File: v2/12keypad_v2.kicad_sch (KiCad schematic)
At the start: 56 parts, among them J1 USB_C_Receptacle_USB2.0, SW1 SW_SPDT, SW10 KEY_MX, SW11 KEY_MX, SW2 KEY_MX, SW3 KEY_MX, SW4 KEY_MX, SW5 KEY_MX, SW6 KEY_MX, SW7 KEY_MX, SW8 KEY_MX, SW9 KEY_MX, U1 RP2040, U2 NCP1117-3.3_SOT223, U3 W25Q128JVS, Y1 12MHz

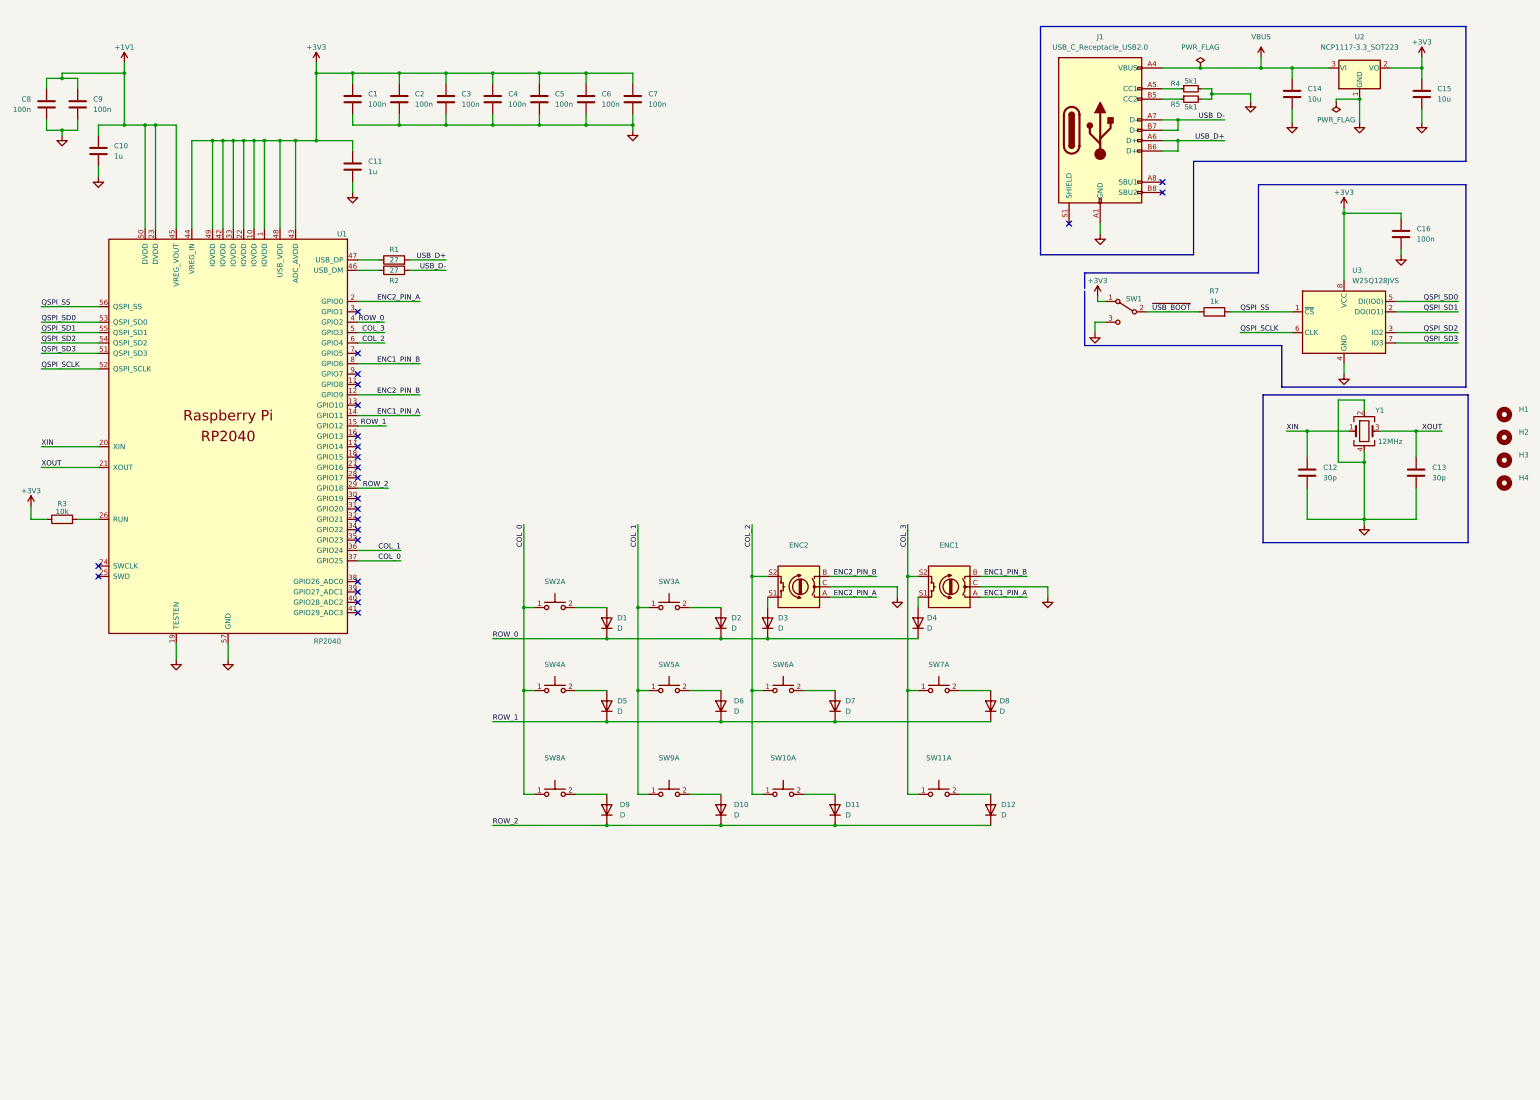
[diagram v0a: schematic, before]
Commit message: general commit
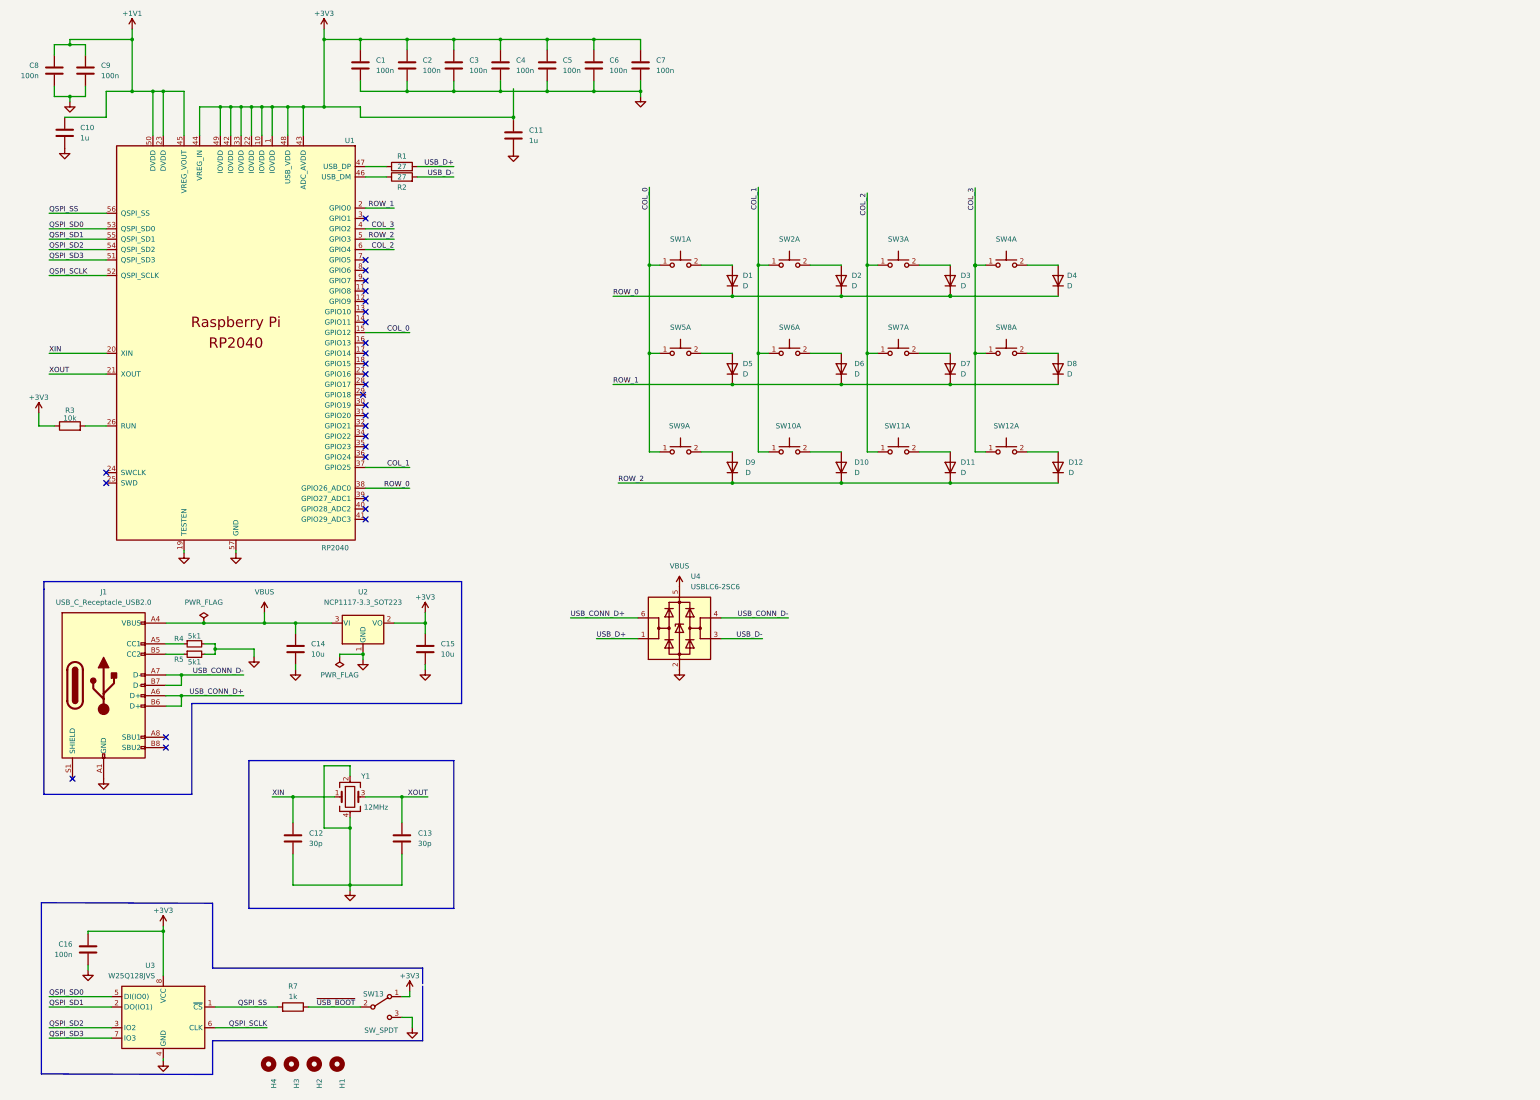
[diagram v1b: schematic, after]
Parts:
- removed ENC1, ENC2: Encoder_Switch, Rotary_Encoder:RotaryEncoder_Alps_EC11E-Switch_Vertical_H20mm, symbol Device:RotaryEncoder_Switch
- added SW1, SW12: KEY_MX, Switch_Keyboard_Cherry_MX:SW_Cherry_MX_PCB_1.00u, symbol keebio:MX_LED
- added U4: USBLC6-2SC6, Package_TO_SOT_SMD:SOT-23-6, symbol Power_Protection:USBLC6-2SC6
- renumbered SW1 to SW13
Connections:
- net ENC2_PIN_A is gone; now on net ROW_1: U1.2 (GPIO0)
- net COL_0: now also SW5.1, SW9.1, U1.15 (GPIO12), SW1.1; no longer SW2.1, SW4.1, SW8.1, U1.37 (GPIO25)
- net COL_1: now also SW10.1, SW2.1, SW6.1, U1.37 (GPIO25); no longer SW3.1, SW5.1, SW9.1, U1.36 (GPIO24)
- net COL_2: now also SW11.1, SW3.1, SW7.1; no longer SW10.1, SW6.1
- net COL_3: now also SW4.1, SW8.1, U1.4 (GPIO2), SW12.1; no longer SW11.1, SW7.1, U1.5 (GPIO3)
- net GND: now also U4.2 (GND)
- net ROW_0: now also U1.38 (GPIO26_ADC0); no longer U1.4 (GPIO2)
- net ROW_1: no longer U1.15 (GPIO12)
- net ROW_2: now also U1.5 (GPIO3); no longer U1.29 (GPIO18)
- net USB_D+: now also U4.1 (I/O1); no longer J1.A6 (D+), J1.B6 (D+)
- net USB_D-: now also U4.3 (I/O2); no longer J1.A7 (D-), J1.B7 (D-)
- net VBUS: now also U4.5 (VBUS)
- net at D4.2 (A): now also SW4.2
- net at D12.2 (A): now also SW12.2; no longer SW11.2
- net at SW3.2: now also D3.2 (A); no longer D2.2 (A)
- net at D8.2 (A): now also SW8.2; no longer SW7.2
- net at D7.2 (A): now also SW7.2; no longer SW6.2
- net at SW10.2: now also D10.2 (A); no longer D11.2 (A)
- net at SW2.2: now also D2.2 (A); no longer D1.2 (A)
- net at D5.2 (A): now also SW5.2; no longer SW4.2
- net at D6.2 (A): now also SW6.2; no longer SW5.2
- net at D9.2 (A): now also SW9.2; no longer SW8.2
- net ENC1_PIN_A: no longer names the net of U1.14 (GPIO11)
- net ENC1_PIN_B: no longer names the net of U1.8 (GPIO6)
- net ENC2_PIN_B: no longer names the net of U1.12 (GPIO9)
- new net: D11.2 (A), SW11.2
- new net: D1.2 (A), SW1.2
- new net USB_CONN_D+: J1.A6 (D+), J1.B6 (D+), U4.6 (I/O1)
- new net USB_CONN_D-: J1.A7 (D-), J1.B7 (D-), U4.4 (I/O2)
- no-connect marks 24 -> 28
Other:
- moved on the sheet: C1, C10, C11, C12, C13, C14, C15, C16, C2, C3, C4, C5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
